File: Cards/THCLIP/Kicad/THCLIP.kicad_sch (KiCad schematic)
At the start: 12 parts, among them J2 Conn_01x03_Pin, J3 Conn_01x05_Pin, K1 Relay_SPDT, U1 RS3K-2424S/H3

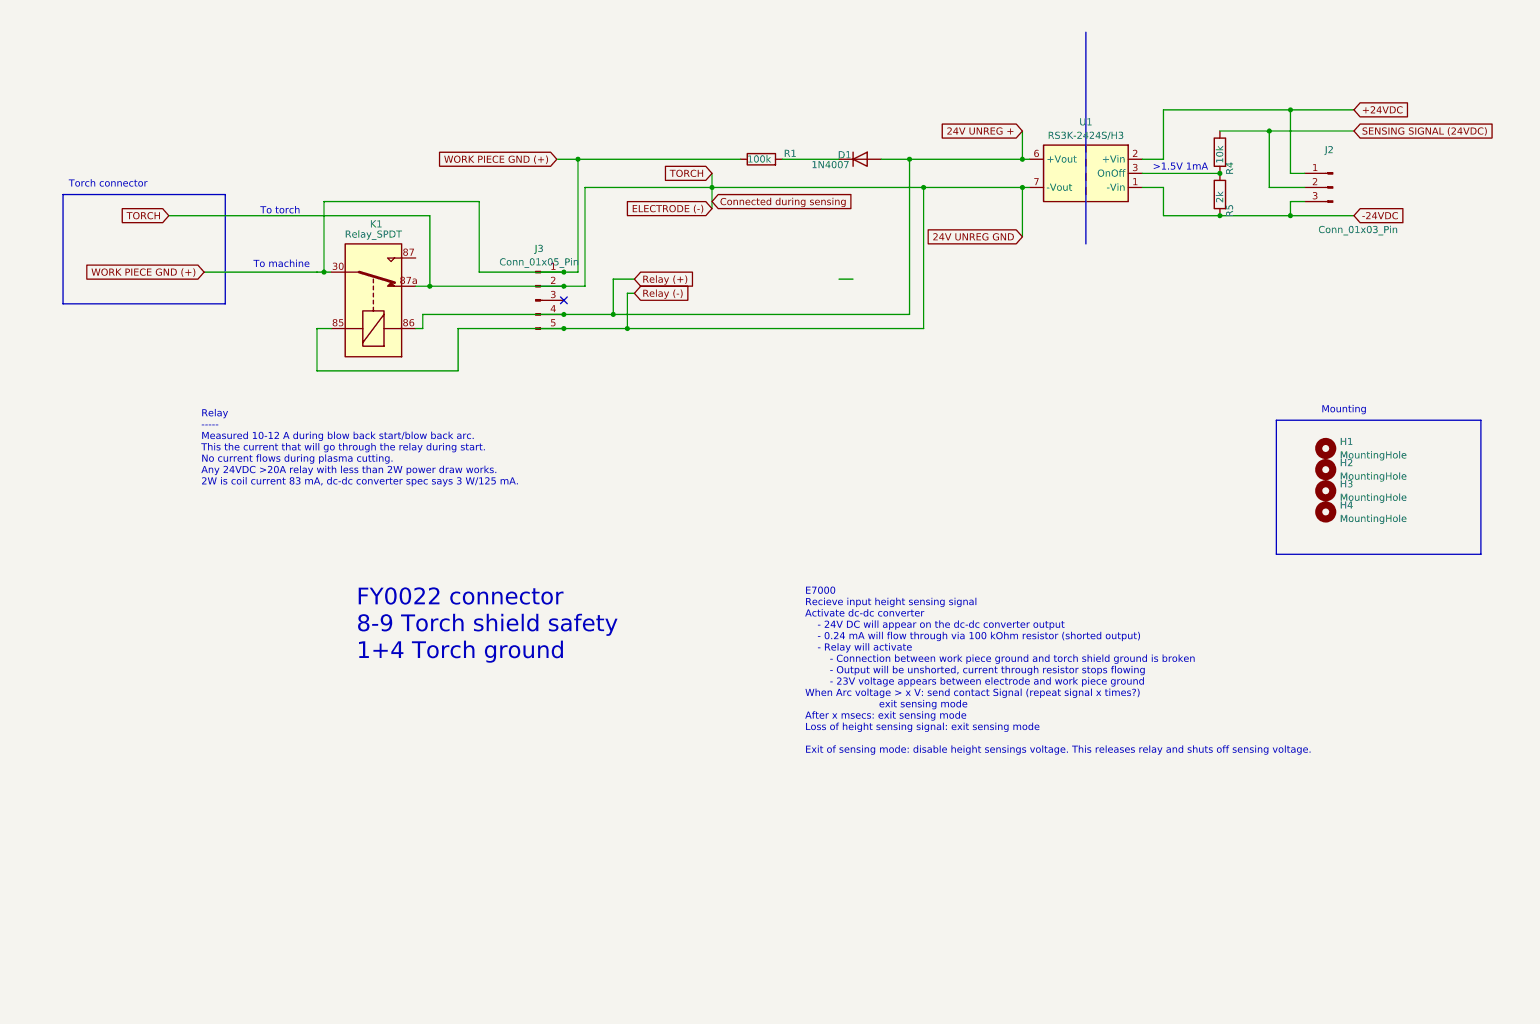
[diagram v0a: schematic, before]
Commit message: Cleaned schematics
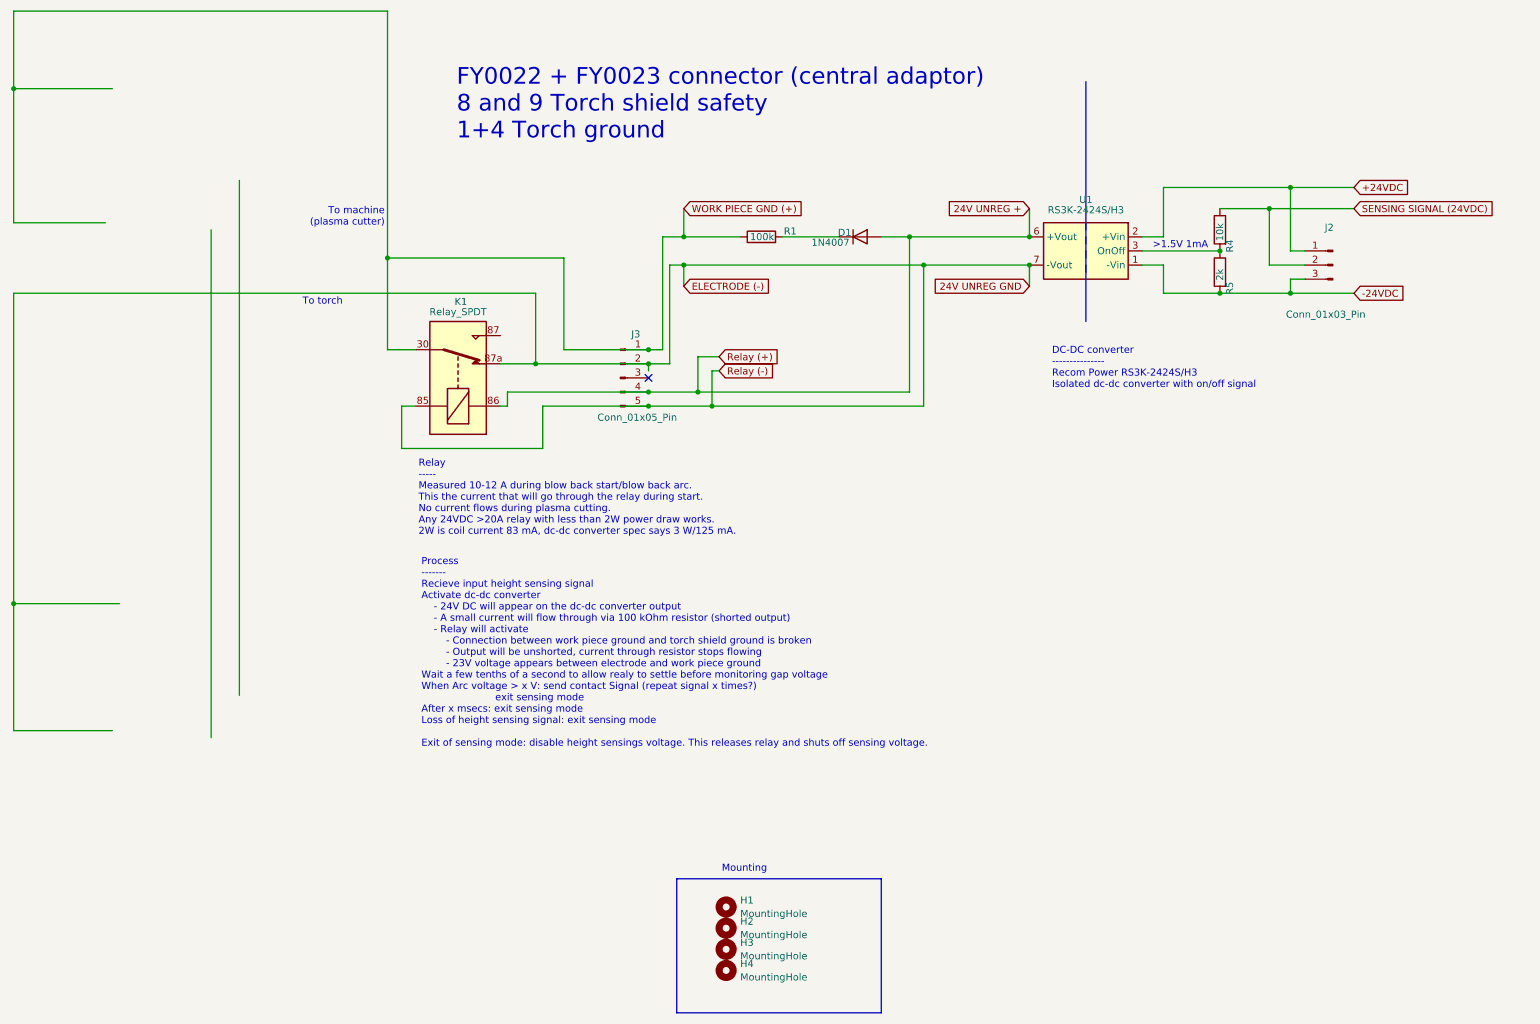
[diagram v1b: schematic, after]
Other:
- note added: "DC-DC converter --------------- Recom Power RS3K-2424S/H3 Isolated dc-dc converter with on/off signal"
- note added: "FY0022 + FY0023 connector (central adaptor) 8 and 9 Torch shield safety 1+4 Torch ground"
- note added: "Process ------- Recieve input height sensing signal Activate dc-dc converter - 24V DC will appear on the dc-dc converter output - A small current will flow through via 100 kOhm resistor (shorted output) - Relay will activate - Connection between work piece ground and torch shield ground is broken - Output will be unshorted, current through resistor stops flowing - 23V voltage appears between elec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"
- note added: "To machine (plasma cutter)"
- note removed: "E7000 Recieve input height sensing signal Activate dc-dc converter - 24V DC will appear on the dc-dc converter output - 0.24 mA will flow through via 100 kOhm resistor (shorted output) - Relay will activate - Connection between work piece ground and torch shield ground is broken - Output will be unshorted, current through resistor stops flowing - 23V voltage appears between electrode and work pie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"
- note removed: "FY0022 connector 8-9 Torch shield safety 1+4 Torch ground"
- note removed: "To machine"
- note removed: "Torch connector"
- moved on the sheet: D1, H1, H2, H3, H4, J2, J3, K1, R1, R4, R5, U1
